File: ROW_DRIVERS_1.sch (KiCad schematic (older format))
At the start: 36 parts, among them Q108 DMG6602, Q109 DMG6602, Q110 SSM3K35AMFV, Q111 SSM3K35AMFV, Q112 SSM3K35AMFV, Q113 SSM3K35AMFV, Q114 DMG6602, Q115 DMG6602, Q116 SSM3K35AMFV, Q117 SSM3K35AMFV, Q118 SSM3K35AMFV, Q119 SSM3K35AMFV

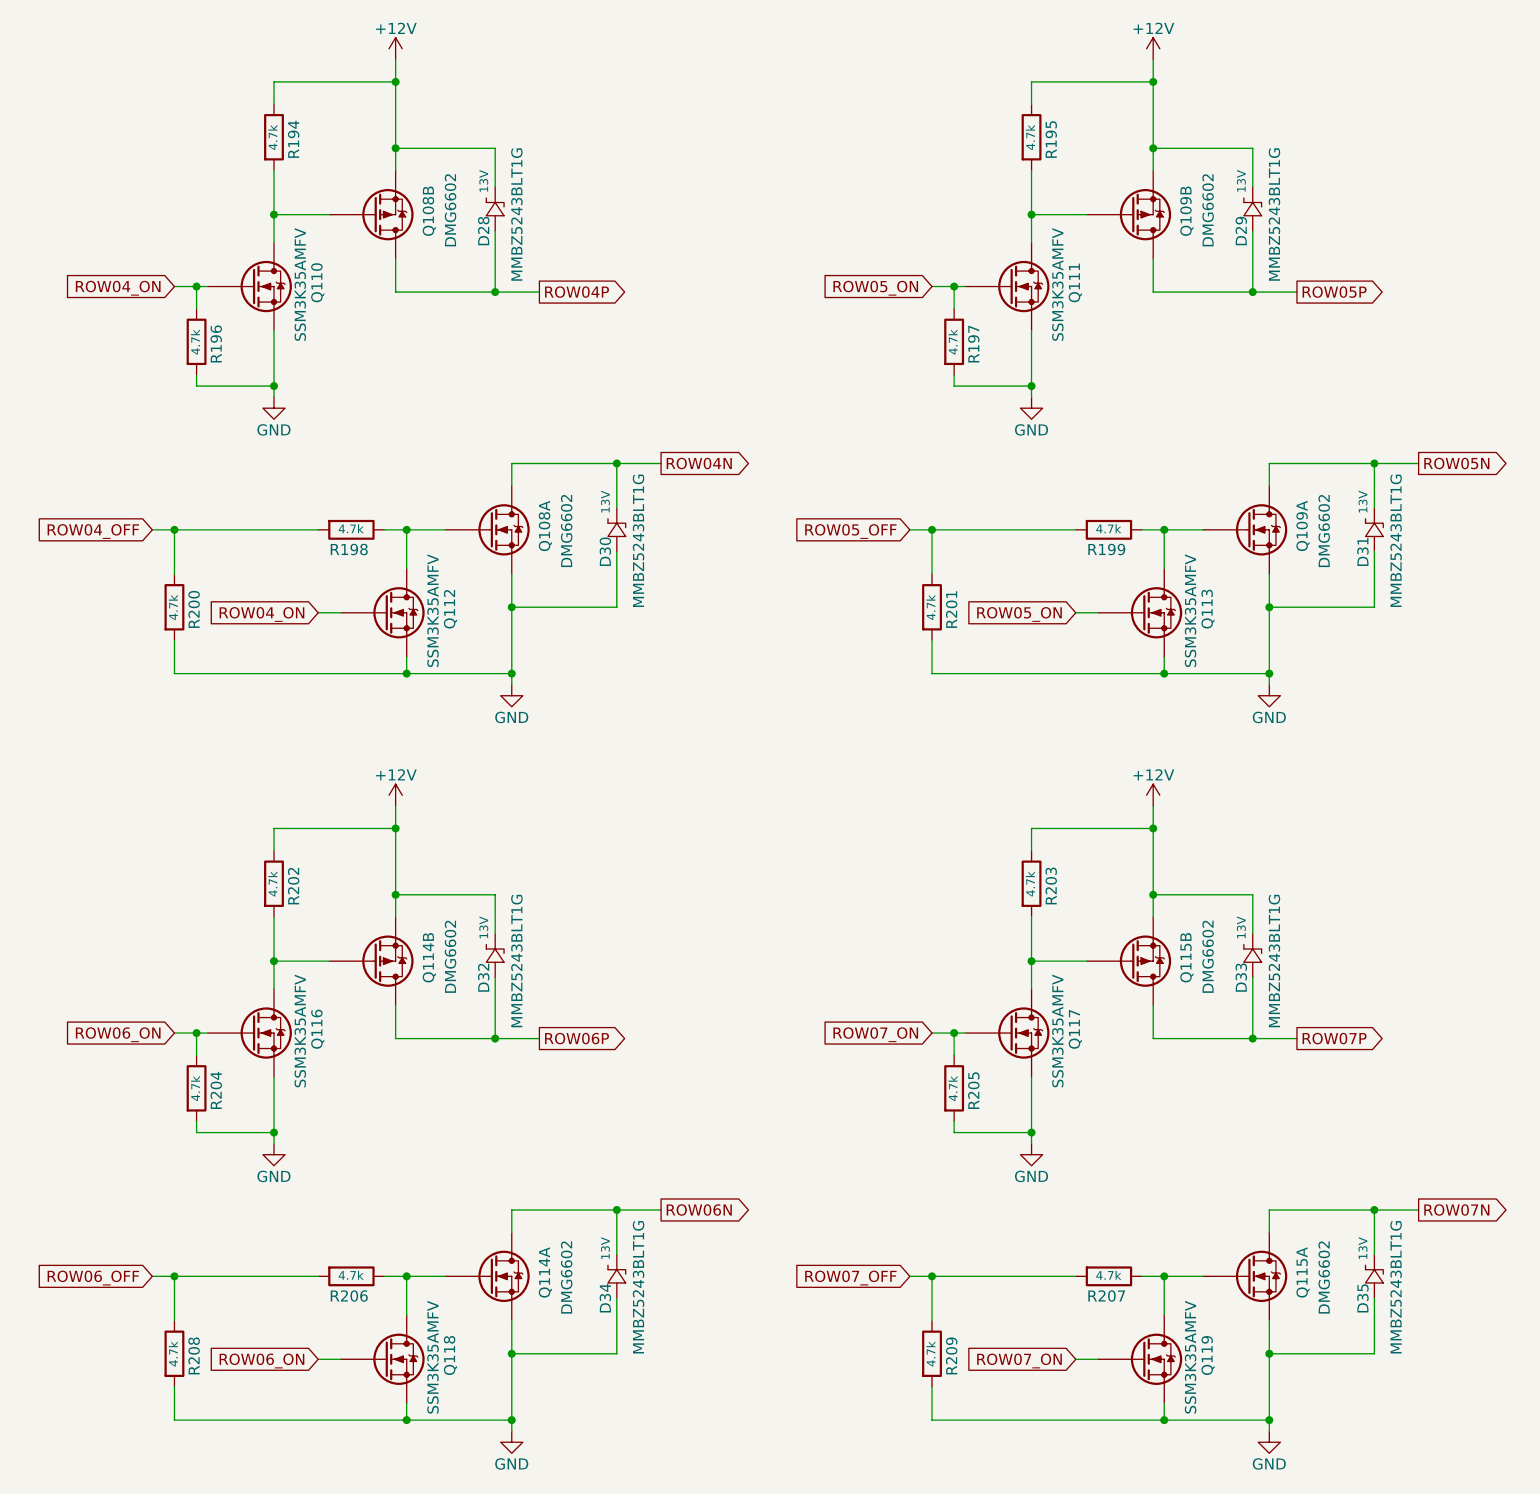
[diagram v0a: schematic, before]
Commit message: automated commit
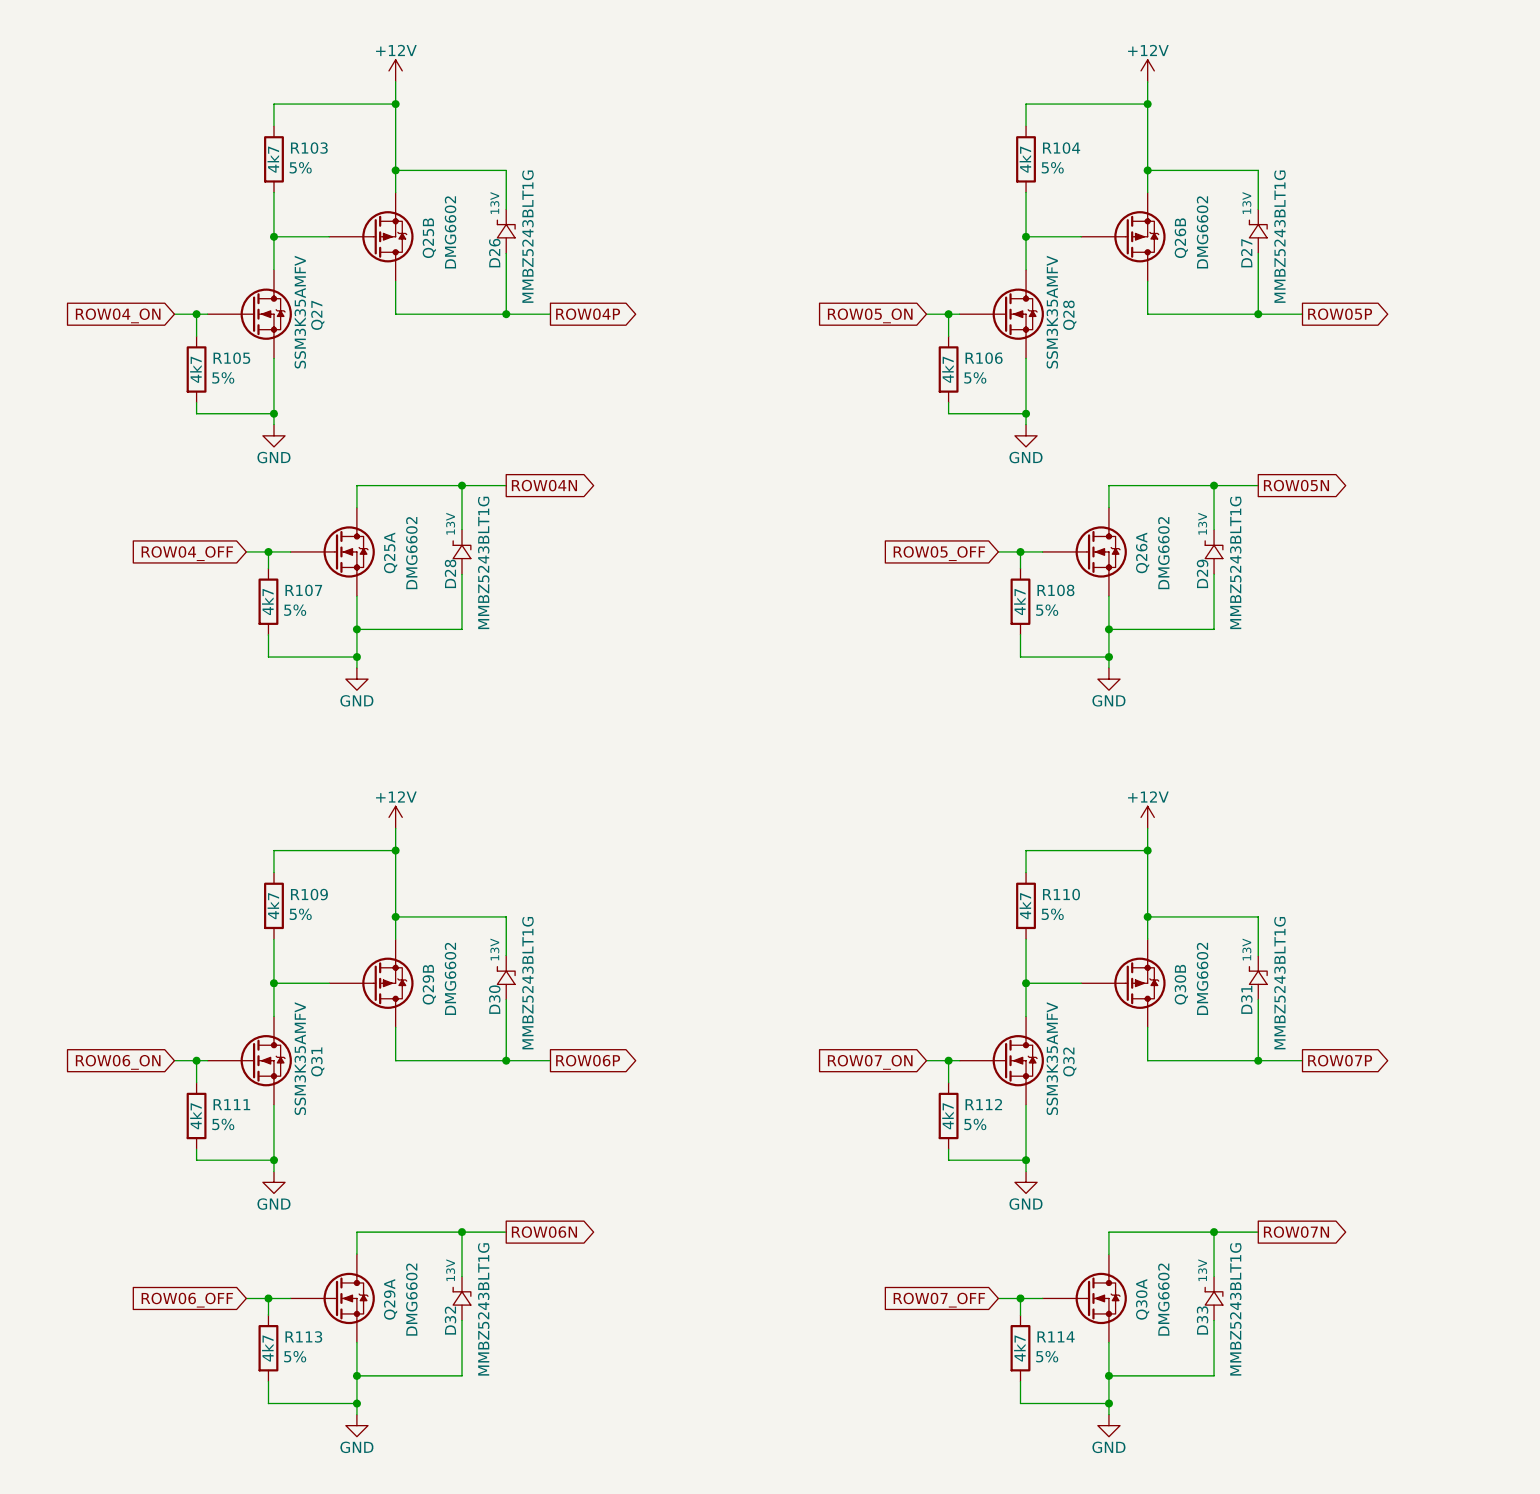
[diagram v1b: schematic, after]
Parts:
- removed D34, D35: MMBZ5243BLT1G, symbol custom:MMBZ5243BLT1G
- removed Q108, Q109, Q114, Q115: DMG6602, Package_TO_SOT_SMD:TSOT-23-6, symbol custom:DMG6602
- removed Q110, Q111, Q112, Q113, Q116, Q117, Q118, Q119: SSM3K35AMFV, symbol custom:SSM3K35AMFV
- removed R194, R195, R196, R197, R198, R199, R200, R201, R202, R203, R204, R205, R206, R207, R208, R209: CRG0603F4K7, Resistor_SMD:R_0603_1608Metric, symbol custom:CRG0603F4K7
- added D26, D27: MMBZ5243BLT1G, symbol custom:MMBZ5243BLT1G
- added Q25, Q26, Q29, Q30: DMG6602, Package_TO_SOT_SMD:TSOT-23-6, symbol custom:DMG6602
- added Q27, Q28, Q31, Q32: SSM3K35AMFV, symbol custom:SSM3K35AMFV
- added R103, R104, R105, R106, R107, R108, R109, R110, R111, R112, R113, R114: CRG0603F4K7, Resistor_SMD:R_0603_1608Metric, symbol custom:CRG0603F4K7
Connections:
- net +12V: now also D30.1 (K), D31.1 (K), D26.1 (K), D27.1 (K), Q25.2 (S), Q26.2 (S), Q29.2 (S), Q30.2 (S), R103.1, R104.1, R109.1, R110.1; no longer D28.1 (K), D29.1 (K), D32.1 (K), D33.1 (K)
- net GND: now also D28.2 (A), D29.2 (A), D32.2 (A), D33.2 (A), Q25.5 (S), Q26.5 (S), Q27.2 (S), Q28.2 (S), Q29.5 (S), Q30.5 (S), Q31.2 (S), Q32.2 (S), R105.2, R106.2, R107.2, R108.2, R111.2, R112.2, R113.2, R114.2; no longer D30.2 (A), D31.2 (A)
- net ROW04N: now also D28.1 (K), Q25.6 (D); no longer D30.1 (K)
- net ROW04P: now also D26.2 (A), Q25.4 (D); no longer D28.2 (A)
- net ROW04_OFF: now also Q25.1 (G), R107.1
- net ROW04_ON: now also Q27.1 (G), R105.1
- net ROW05N: now also D29.1 (K), Q26.6 (D); no longer D31.1 (K)
- net ROW05P: now also D27.2 (A), Q26.4 (D); no longer D29.2 (A)
- net ROW05_OFF: now also Q26.1 (G), R108.1
- net ROW05_ON: now also Q28.1 (G), R106.1
- net ROW06N: now also D32.1 (K), Q29.6 (D)
- net ROW06P: now also D30.2 (A), Q29.4 (D); no longer D32.2 (A)
- net ROW06_OFF: now also Q29.1 (G), R113.1
- net ROW06_ON: now also Q31.1 (G), R111.1
- net ROW07N: now also D33.1 (K), Q30.6 (D)
- net ROW07P: now also D31.2 (A), Q30.4 (D); no longer D33.2 (A)
- net ROW07_OFF: now also Q30.1 (G), R114.1
- net ROW07_ON: now also Q32.1 (G), R112.1
- new net: Q26.3 (G), Q28.3 (D), R104.2
- new net: Q30.3 (G), Q32.3 (D), R110.2
- new net: Q29.3 (G), Q31.3 (D), R109.2
- new net: Q25.3 (G), Q27.3 (D), R103.2
